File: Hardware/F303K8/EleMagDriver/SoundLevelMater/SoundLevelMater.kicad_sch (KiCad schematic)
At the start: 10 parts, among them J1 Conn_01x03_Socket, J2 Conn_02x10_Odd_Even, J3 Barrel_Jack, U1 LM3914N

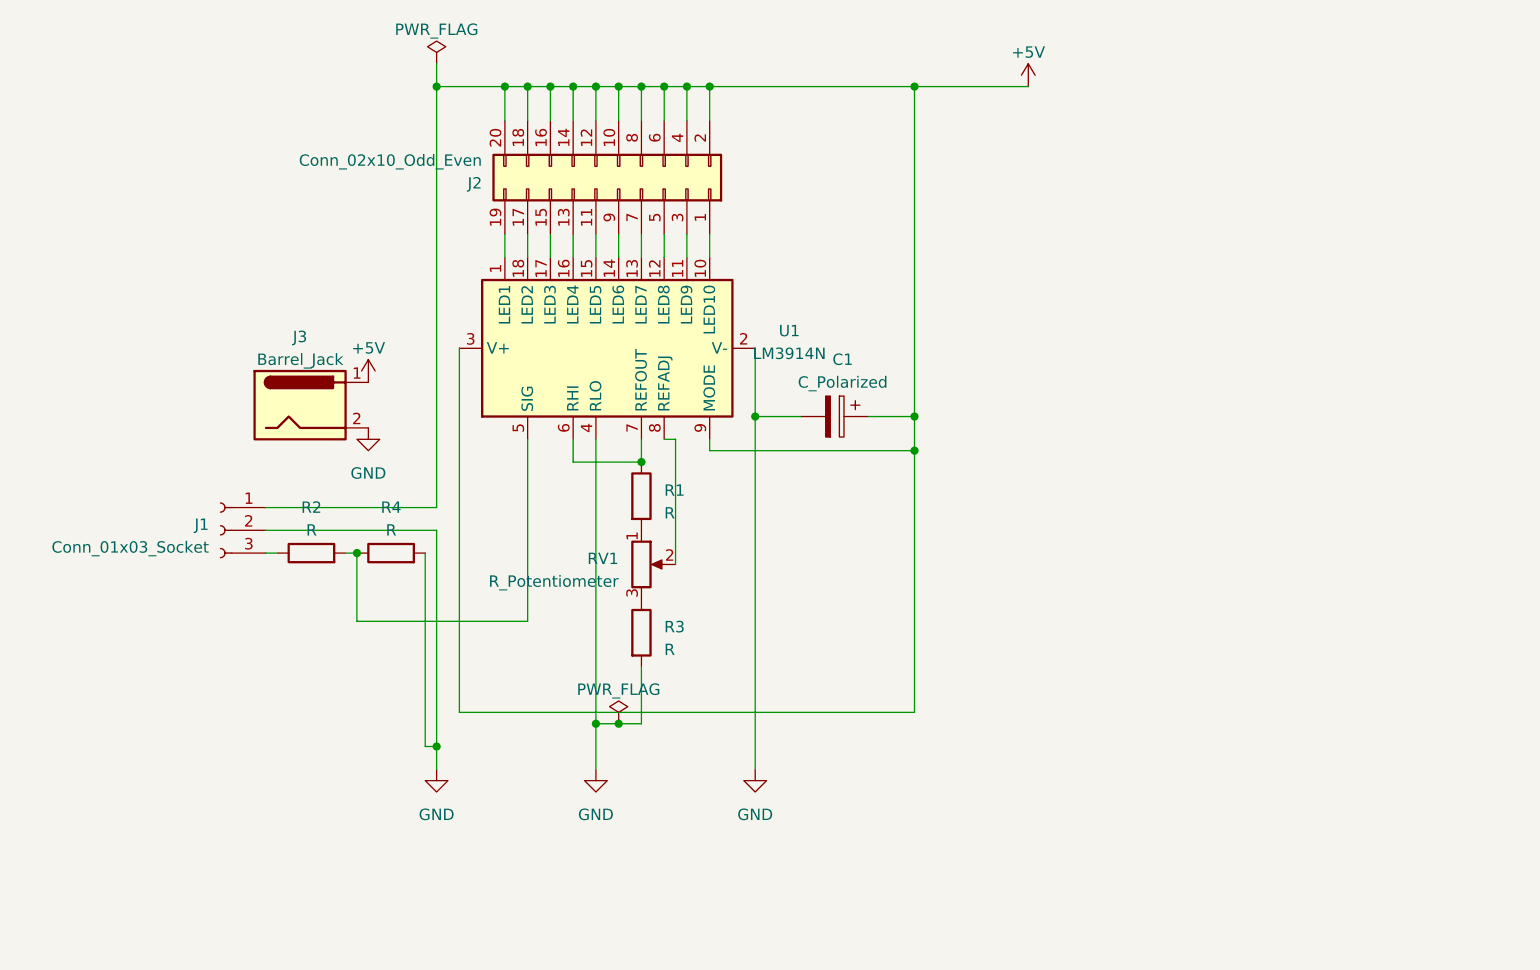
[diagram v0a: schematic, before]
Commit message: edit circuit
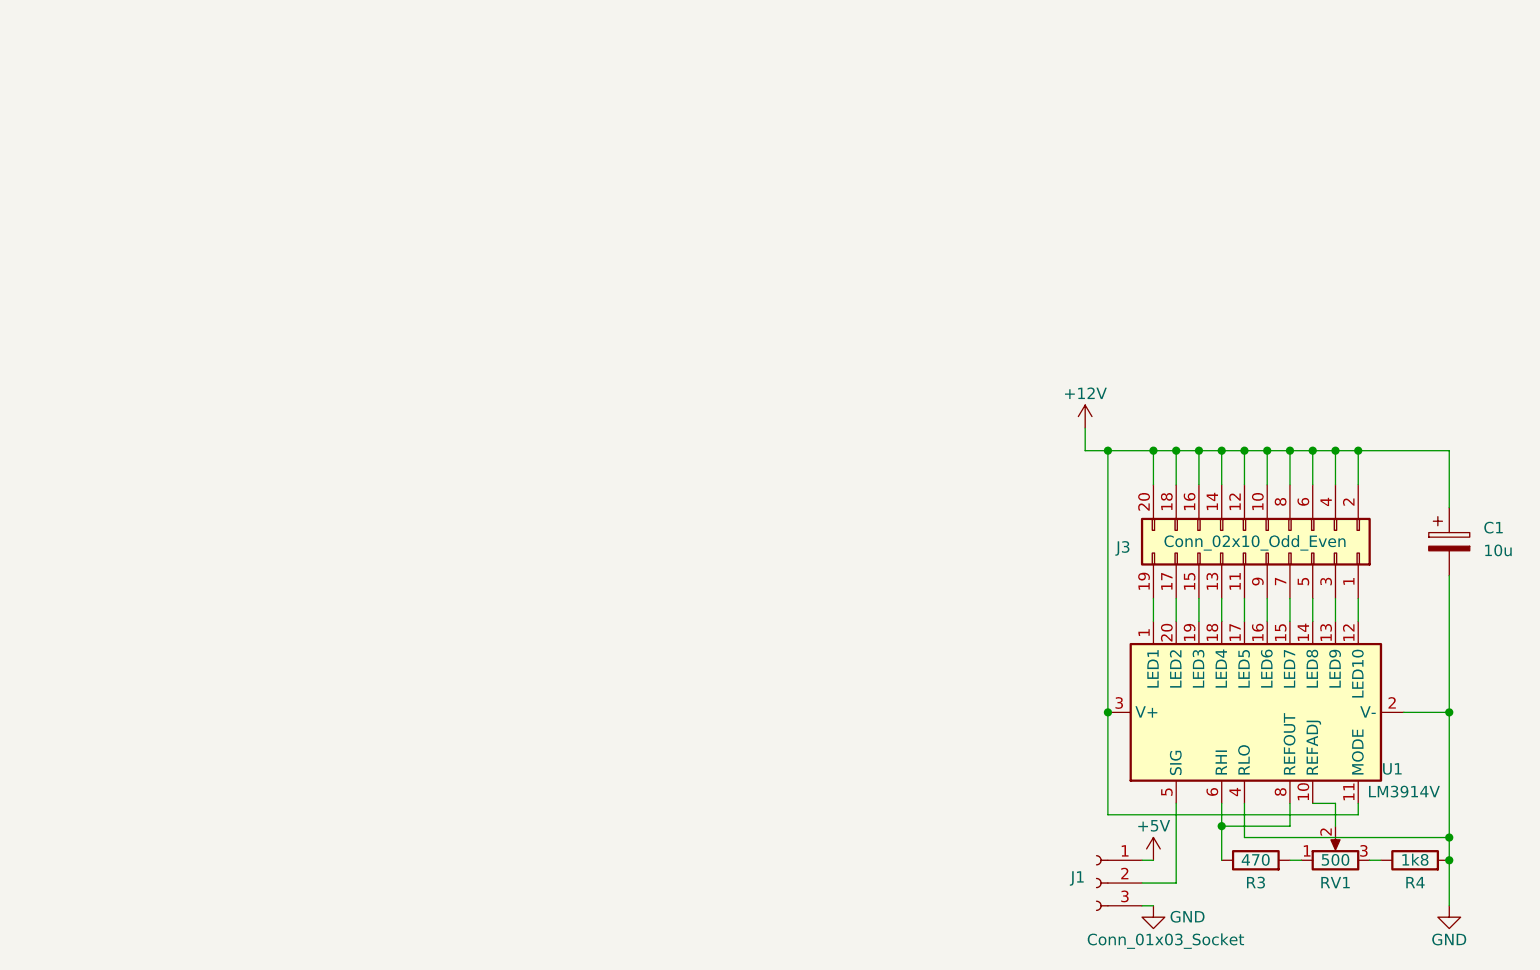
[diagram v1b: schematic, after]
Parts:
- removed J2: Conn_02x10_Odd_Even, Connector_PinSocket_2.00mm:PinSocket_2x10_P2.00mm_Vertical, symbol Connector_Generic:Conn_02x10_Odd_Even
- removed J3: Barrel_Jack, Connector_BarrelJack:BarrelJack_SwitchcraftConxall_RAPC10U_Horizontal, symbol Connector:Barrel_Jack
- removed R1, R2: R, Resistor_SMD:R_0402_1005Metric, symbol Device:R
- removed U1: LM3914N, Package_DIP:DIP-18_W7.62mm, symbol Driver_LED:LM3914N
- added J3: Conn_02x10_Odd_Even, Connector_PinSocket_2.00mm:PinSocket_2x10_P2.00mm_Horizontal, symbol Connector_Generic:Conn_02x10_Odd_Even
- added U1: LM3914V, Package_LCC:PLCC-20, symbol Driver_LED:LM3914V
- C1: value C_Polarized -> 10u
- R3: value R -> 470
- R4: value R -> 1k8
- RV1: value R_Potentiometer -> 500
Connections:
- net +5V: no longer C1.1
- net GND: now also J1.3 (Pin_3), U1.2 (V-), U1.4 (RLO); no longer J1.2 (Pin_2), R3.2
- net at RV1.1: now also R3.2
- net at RV1.2: now also U1.10 (REFADJ)
- net at RV1.3: now also R4.1; no longer R3.1
- new net: J1.2 (Pin_2), U1.5 (SIG)
- new net: R3.1, U1.6 (RHI), U1.8 (REFOUT)
- new net: J3.19 (Pin_19), U1.1 (LED1)
- new net: J3.1 (Pin_1), U1.12 (LED10)
- new net: J3.3 (Pin_3), U1.13 (LED9)
- new net: J3.5 (Pin_5), U1.14 (LED8)
- new net: J3.7 (Pin_7), U1.15 (LED7)
- new net: J3.9 (Pin_9), U1.16 (LED6)
- new net: J3.11 (Pin_11), U1.17 (LED5)
- new net: J3.13 (Pin_13), U1.18 (LED4)
- new net: J3.15 (Pin_15), U1.19 (LED3)
- new net: J3.17 (Pin_17), U1.20 (LED2)
- new net +12V: C1.1, J3.10 (Pin_10), J3.12 (Pin_12), J3.14 (Pin_14), J3.16 (Pin_16), J3.18 (Pin_18), J3.2 (Pin_2), J3.20 (Pin_20), J3.4 (Pin_4), J3.6 (Pin_6), J3.8 (Pin_8), U1.11 (MODE), U1.3 (V+)
